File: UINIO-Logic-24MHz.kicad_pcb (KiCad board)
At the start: 2 copper layers, 48.8 x 25.5 mm, 51 parts, among them J1 Conn_01x10_Male, U1 AT24CS64-XHM, U2 74HC245C, U3 ME6211C33M5G-N, U4 CY7C68013A-56LTX, Y1 24MHz

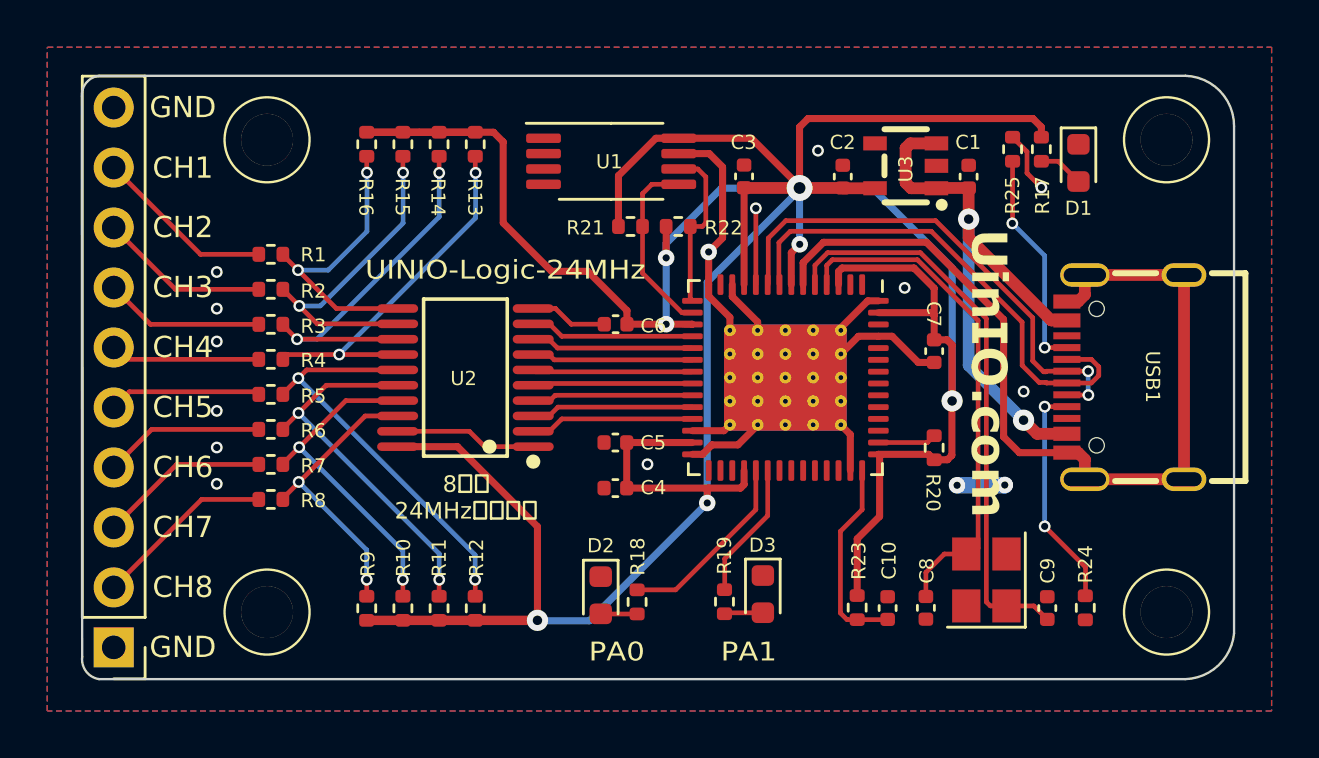
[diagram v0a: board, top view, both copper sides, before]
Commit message: Prepare UINIO-Logic-24MHz version 3.0.0.
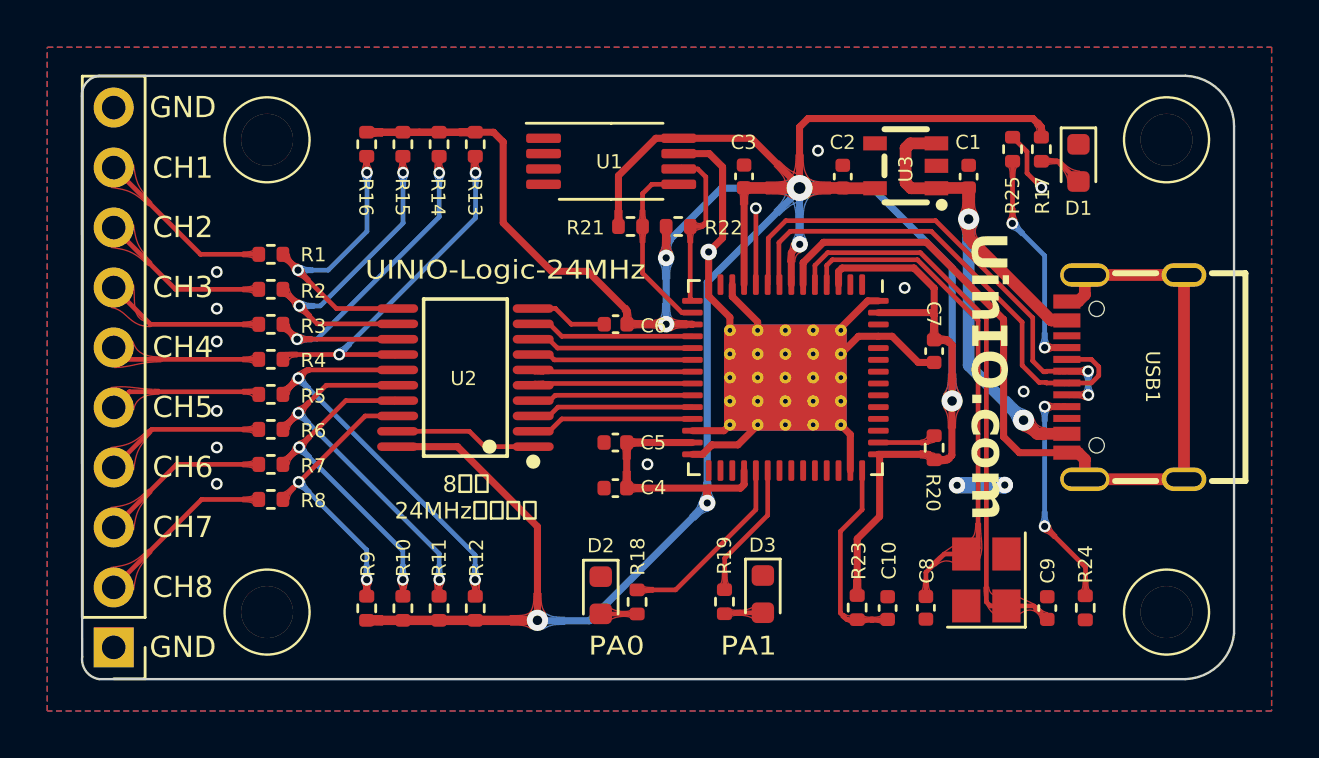
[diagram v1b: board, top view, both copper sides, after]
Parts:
- moved ? 0.12 mm to (144.7, 118.7)
